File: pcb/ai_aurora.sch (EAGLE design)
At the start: 19 parts, among them IC1 ATTINY85-DIP, J1 1X02ST, J2 2X03

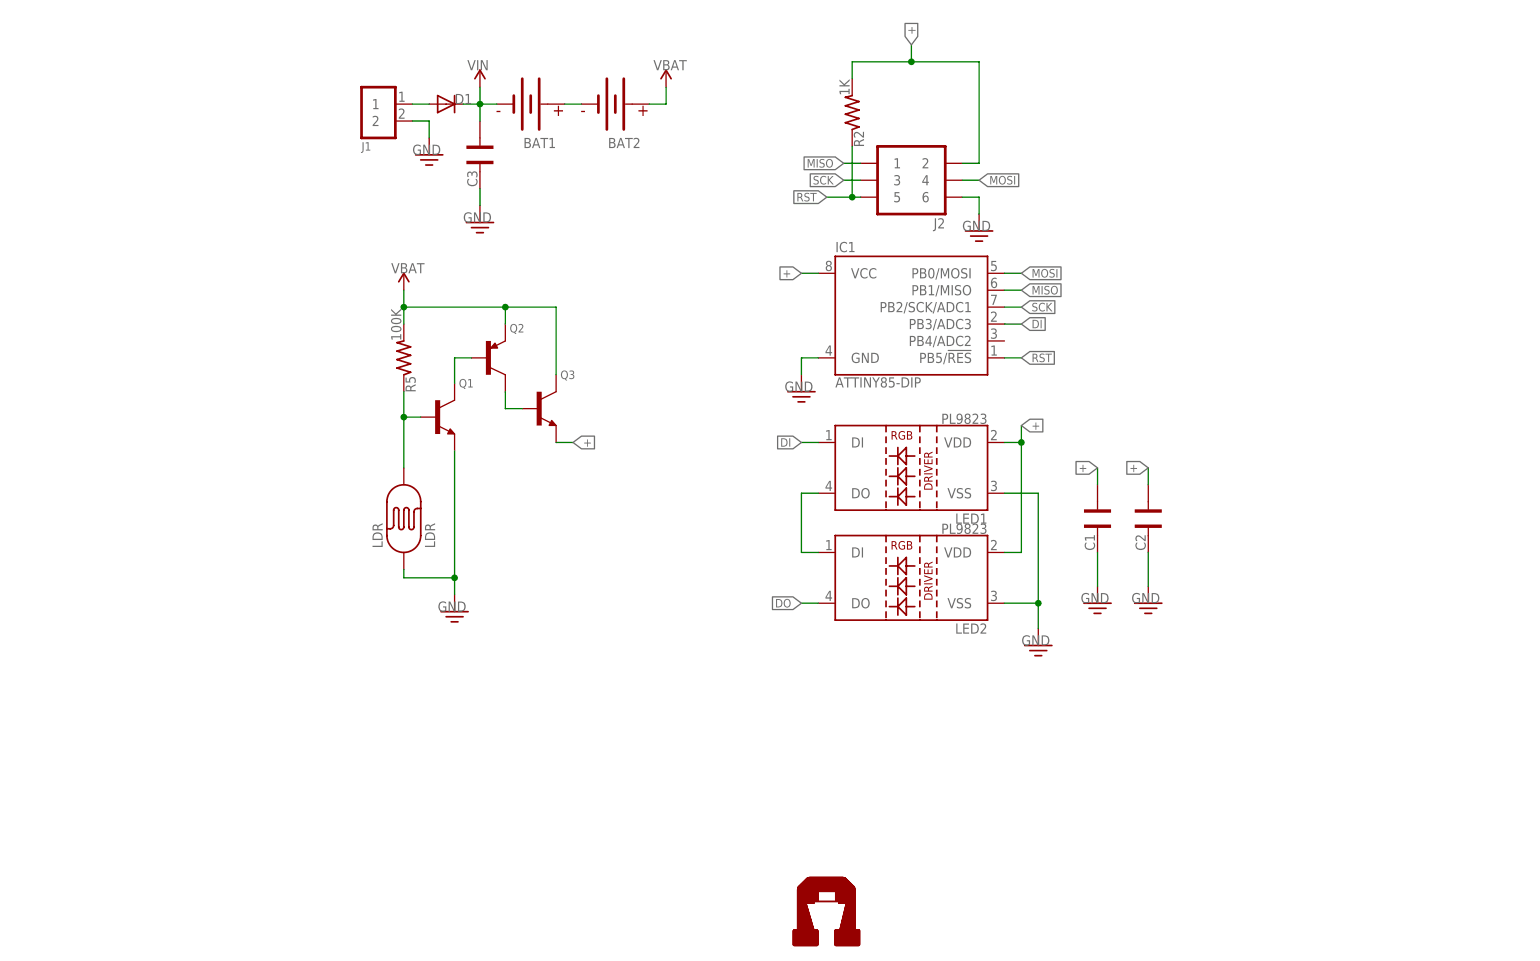
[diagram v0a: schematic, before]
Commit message: updating firmware and pcb
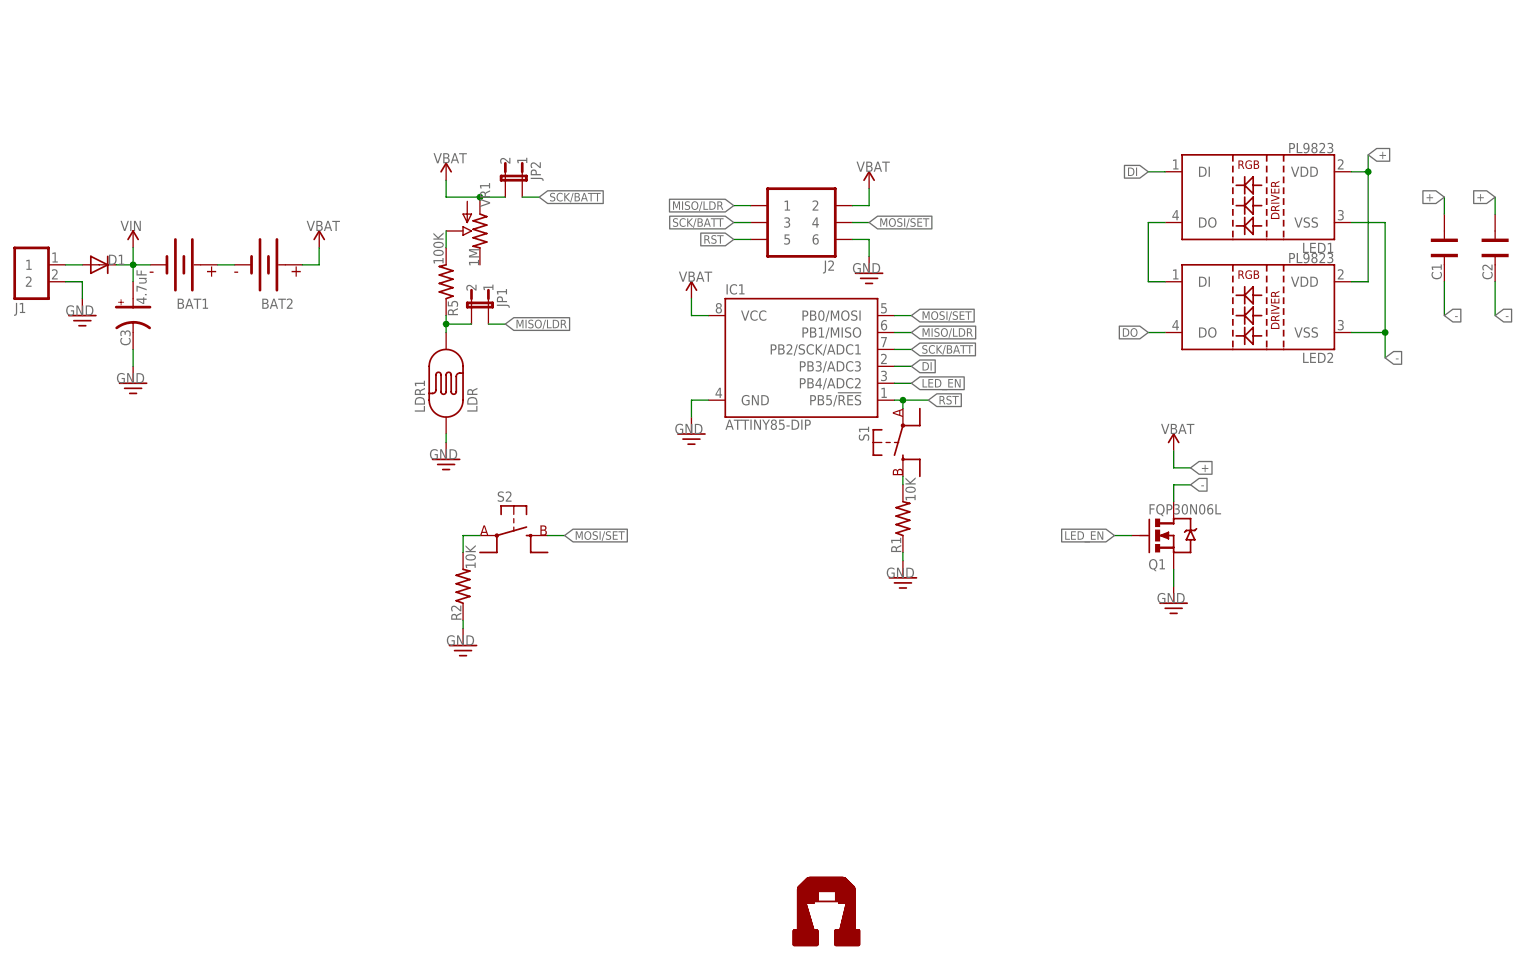
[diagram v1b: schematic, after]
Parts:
- removed LDR: LDR-PTH, Ai_Sensors:LDR-PTH
- removed Q2: (no value), Ai_DiscreteSemis:TRANSISTOR-PNP
- removed Q3: (no value), Ai_DiscreteSemis:TRANSISTOR-NPN
- added JP1, JP2: 1X02-PJ, Ai_Connectors:1X02-PJ
- added LDR1: LDR-PTH, Ai_Sensors:LDR-PTH
- added R1: 10K, Ai_Passives:RESAXIAL-0.4
- added S1, S2: SW-SPSTTH06X06, Ai_Electromechanical:SW-SPSTTH06X06
- added VR1: 1M, Ai_Passives:POT05X05
- C3: value (none) -> 4.7uF; device Ai_Passives:CAP025X050 -> Ai_Passives:CAP-POL025X50
- Q1: value (none) -> FQP30N06L; device Ai_DiscreteSemis:TRANSISTOR-NPN -> Ai_DiscreteSemis:FET-NMOS-FQP30N06L
- R2: value 1K -> 10K
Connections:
- net MOSI renamed MOSI/SET
- removed net MISO: IC1.PB1/MISO, J2.1
- removed net N$10: LDR.P$2, Q1.B, R5.1
- removed net N$13: Q1.C, Q2.B
- removed net SCK: IC1.PB2/SCK/ADC1, J2.3
- new net -: C1.2, C2.2, LED1.VSS, LED2.VSS, Q1.D
- new net LED_EN: IC1.PB4/ADC2, Q1.G
- new net MISO/LDR: IC1.PB1/MISO, J2.1, JP1.1
- new net N$3: R1.2, S1.B@1
- new net N$5: R2.2, S2.A@1
- new net N$6: R5.2, VR1.S
- new net N$7: JP1.2, LDR1.P$2, R5.1
- new net SCK/BATT: IC1.PB2/SCK/ADC1, J2.3, JP2.1
- net +: no longer IC1.VCC, J2.2, Q2.C, Q3.B, Q3.E, R2.2
- net GND: now also C3.C, LDR1.P$1, Q1.S, R1.1, R2.1; no longer C1.2, C2.2, C3.2, LDR.P$1, LED1.VSS, LED2.VSS, Q1.E
- net RST: now also S1.A@1; no longer R2.1
- net VBAT: now also IC1.VCC, J2.2, JP2.2, VR1.A; no longer Q2.E, Q3.C, R5.2
- net VIN: now also C3.A; no longer C3.1
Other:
- moved on the sheet: BAT1, BAT2, C1, C2, D1, IC1, J1, J2, LED1, LED2, R2, R5
